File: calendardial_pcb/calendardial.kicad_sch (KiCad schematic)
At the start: 16 parts, among them J1 01x40 FFC Socket, P1 USB_C_Plug_USB2.0, U1 ESP32-S3-WROOM-1-N8R2, U2 TPS61169DCKR, U3 AP2112K-3.3, U4 FT232RL

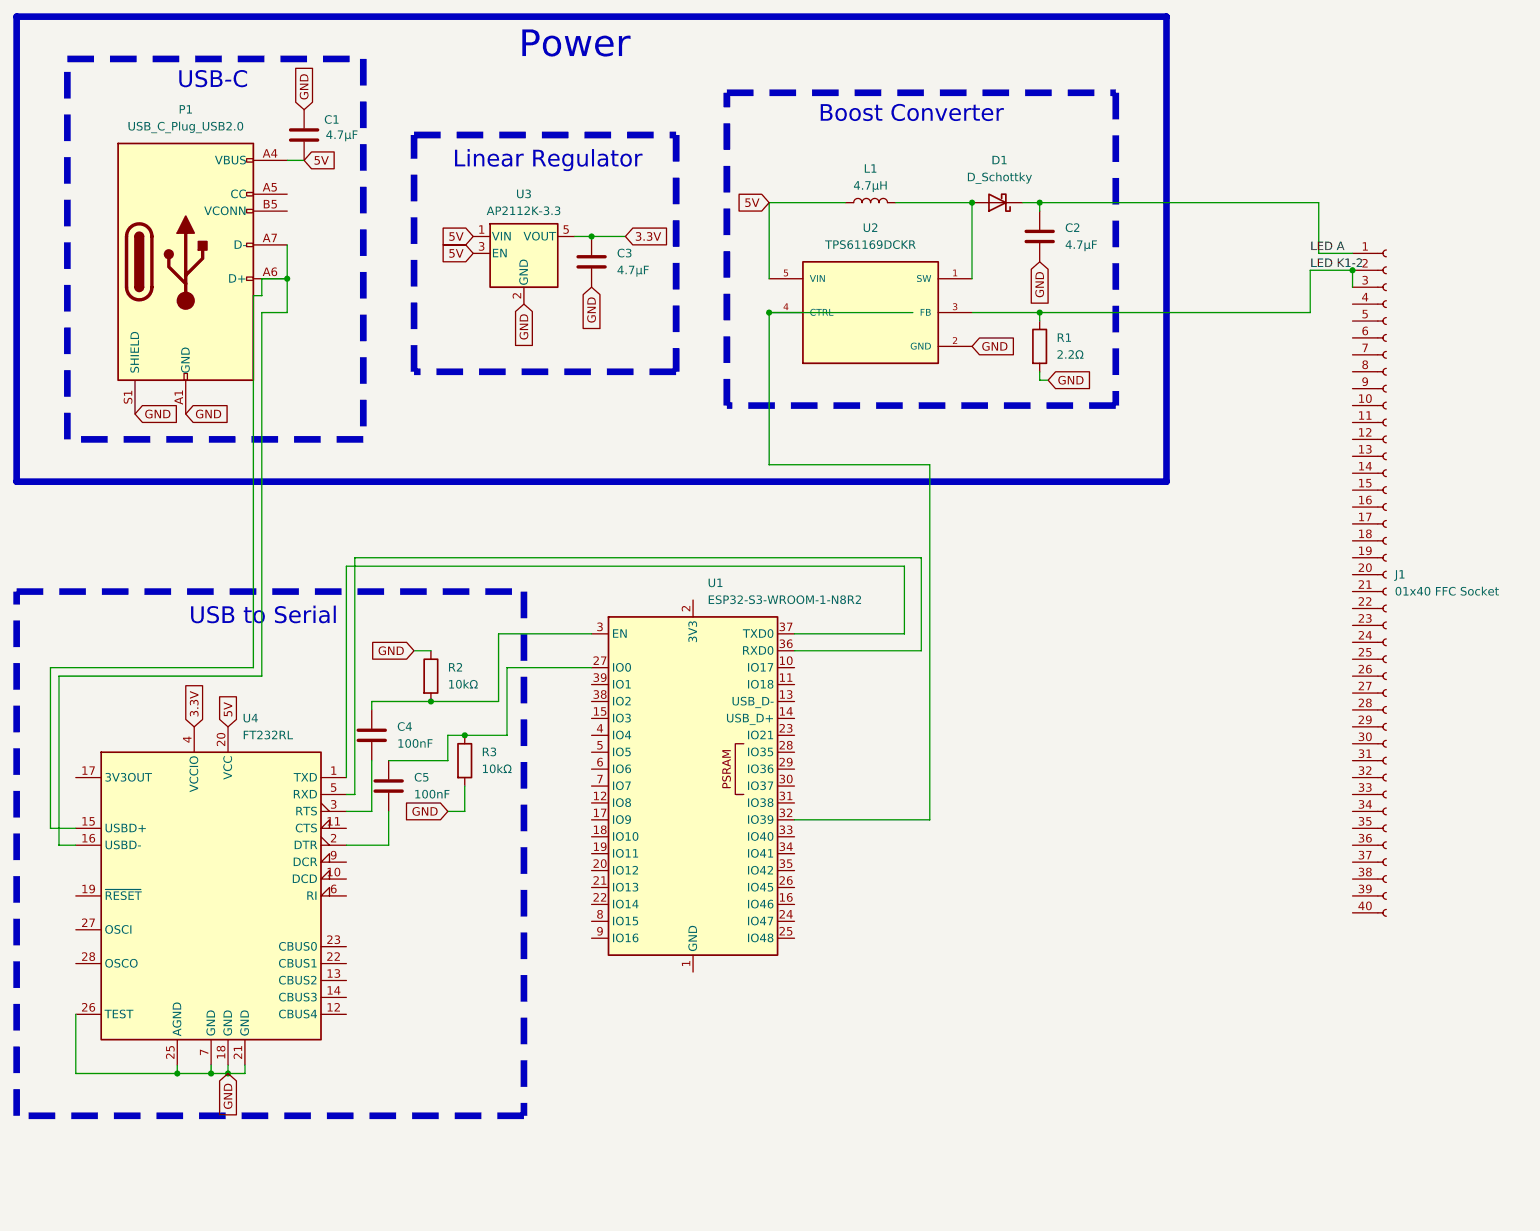
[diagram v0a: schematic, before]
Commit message: e
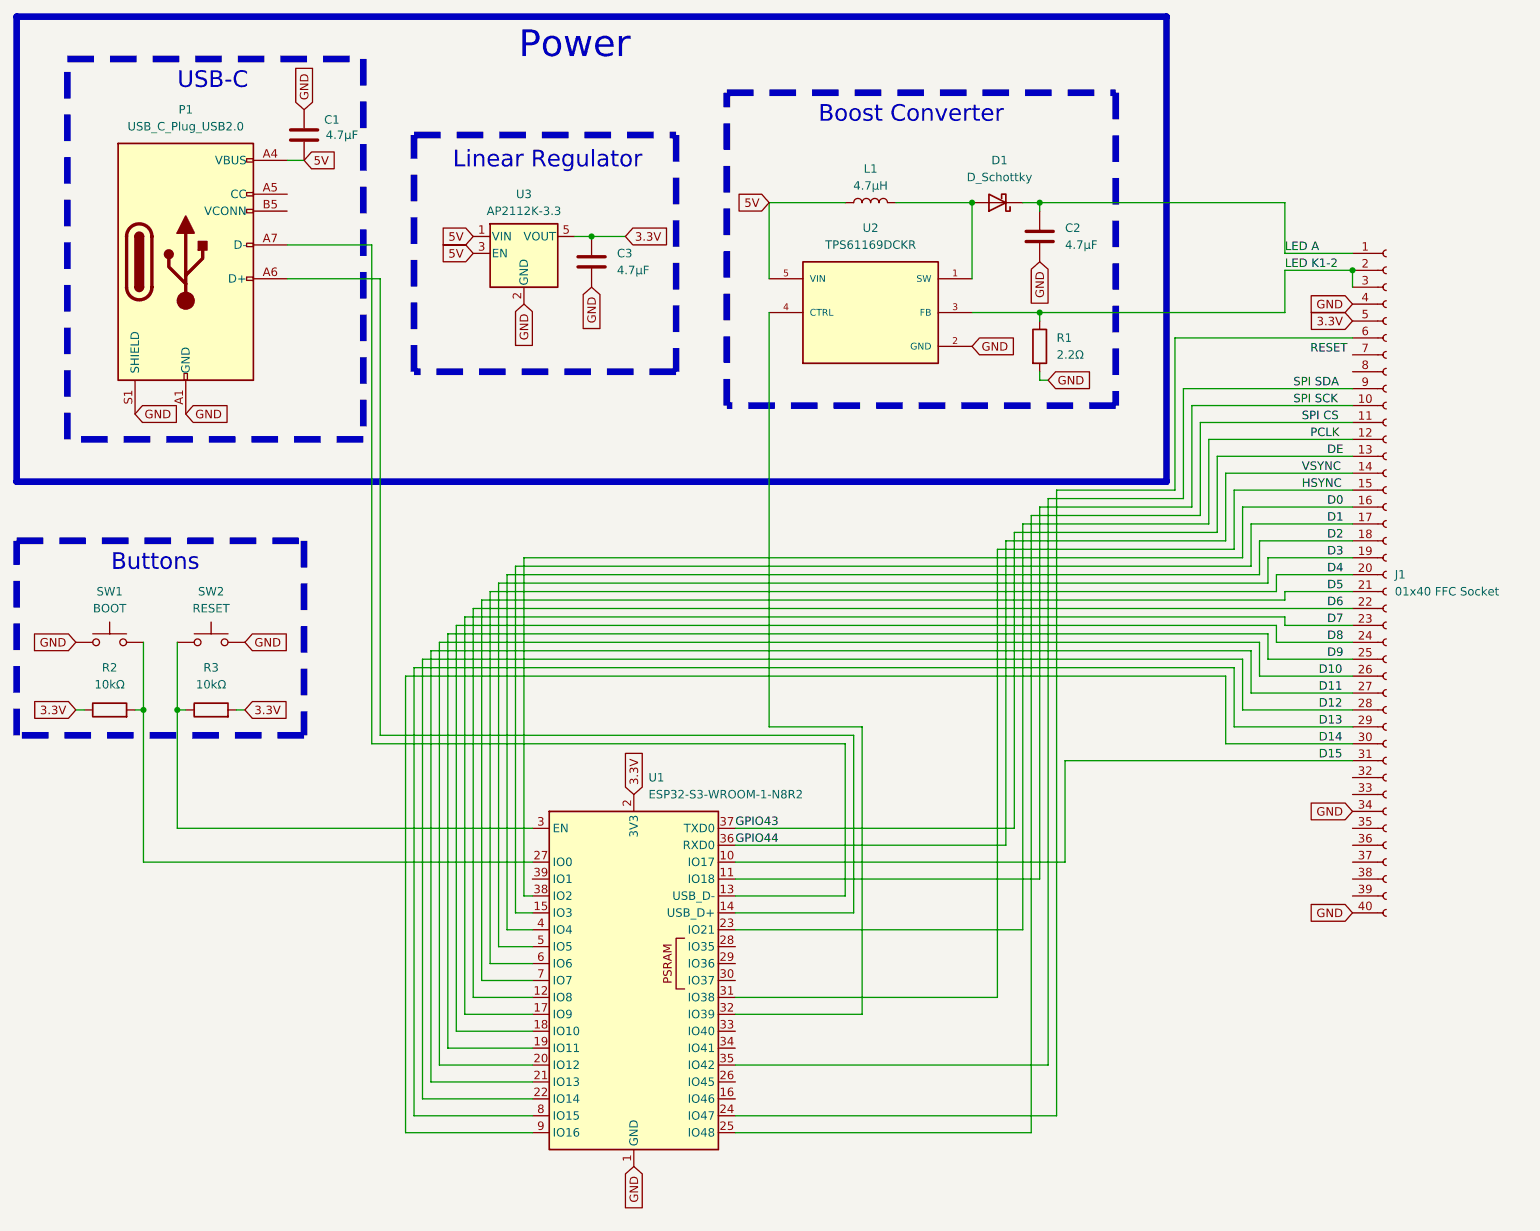
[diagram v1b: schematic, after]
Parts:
- removed C4, C5: 100nF, symbol Device:C
- removed U4: FT232RL, Package_SO:SSOP-28_5.3x10.2mm_P0.65mm, symbol Interface_USB:FT232RL
- added SW1: BOOT, symbol Switch:SW_Push
- added SW2: RESET, symbol Switch:SW_Push
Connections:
- net 3.3V: now also J1.5 (Pin_5), R2.1, R3.2, U1.2 (3V3)
- net GND: now also J1.34 (Pin_34), J1.4 (Pin_4), J1.40 (Pin_40), U1.1 (GND), U1.40 (GND), U1.41 (GND), SW1.1, SW2.2; no longer R2.1, R3.2
- net LED A: now also C2.1, D1.1 (K), J1.1 (Pin_1)
- net at U1.3 (EN): now also R3.1, SW2.1; no longer R2.2
- net at U1.27 (IO0): now also R2.2, SW1.2; no longer R3.1
- net D15: now reaches U1.10 (IO17)
- net D15: now also J1.31 (Pin_31)
- net SPI SCK: now reaches U1.11 (IO18)
- net SPI SCK: now also J1.10 (Pin_10)
- net D6: now reaches U1.12 (IO8)
- net D6: now also J1.22 (Pin_22)
- net at U1.13 (USB_D-): now also P1.A7 (D-)
- net at U1.14 (USB_D+): now also P1.A6 (D+)
- net D1: now reaches U1.15 (IO3)
- net D1: now also J1.17 (Pin_17)
- net D7: now reaches U1.17 (IO9)
- net D7: now also J1.23 (Pin_23)
- net D8: now reaches U1.18 (IO10)
- net D8: now also J1.24 (Pin_24)
- net D9: now reaches U1.19 (IO11)
- net D9: now also J1.25 (Pin_25)
- net D10: now reaches U1.20 (IO12)
- net D10: now also J1.26 (Pin_26)
- net D11: now reaches U1.21 (IO13)
- net D11: now also J1.27 (Pin_27)
- net D12: now reaches U1.22 (IO14)
- net D12: now also J1.28 (Pin_28)
- net PCLK: now reaches U1.23 (IO21)
- net PCLK: now also J1.12 (Pin_12)
- net at U1.24 (IO47): now also J1.6 (Pin_6)
- net SPI CS: now reaches U1.25 (IO48)
- net SPI CS: now also J1.11 (Pin_11)
- net HSYNC: now reaches U1.31 (IO38)
- net HSYNC: now also J1.15 (Pin_15)
- net SPI SDA: now reaches U1.35 (IO42)
- net SPI SDA: now also J1.9 (Pin_9)
- net GPIO44: now reaches U1.36 (RXD0)
- net GPIO44: now also J1.14 (Pin_14)
- net DE: now reaches U1.37 (TXD0)
- net DE: now also J1.13 (Pin_13)
- net D0: now reaches U1.38 (IO2)
- net D0: now also J1.16 (Pin_16)
- net D2: now reaches U1.4 (IO4)
- net D2: now also J1.18 (Pin_18)
- net D3: now reaches U1.5 (IO5)
- net D3: now also J1.19 (Pin_19)
- net D4: now reaches U1.6 (IO6)
- net D4: now also J1.20 (Pin_20)
- net D5: now reaches U1.7 (IO7)
- net D5: now also J1.21 (Pin_21)
- net D13: now reaches U1.8 (IO15)
- net D13: now also J1.29 (Pin_29)
- net D14: now reaches U1.9 (IO16)
- net D14: now also J1.30 (Pin_30)
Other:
- note added: "Buttons"
- note removed: "USB to Serial"
- moved on the sheet: U1
